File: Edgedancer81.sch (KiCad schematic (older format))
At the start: 17 parts, among them SW1 SW_Push, SW2 Rotary_Encoder_Switch, U1 ATmega32U4-AU, Y1 16MHz

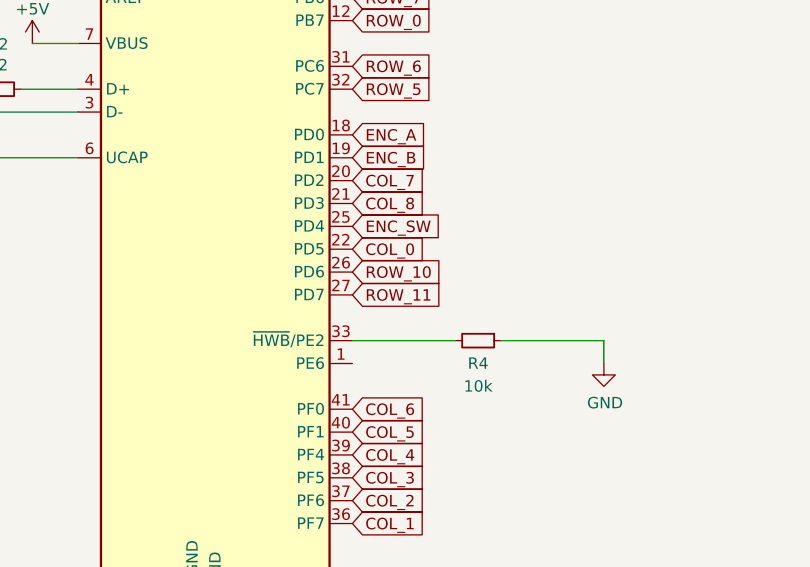
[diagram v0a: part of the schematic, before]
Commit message: silkscreen and bugfixes
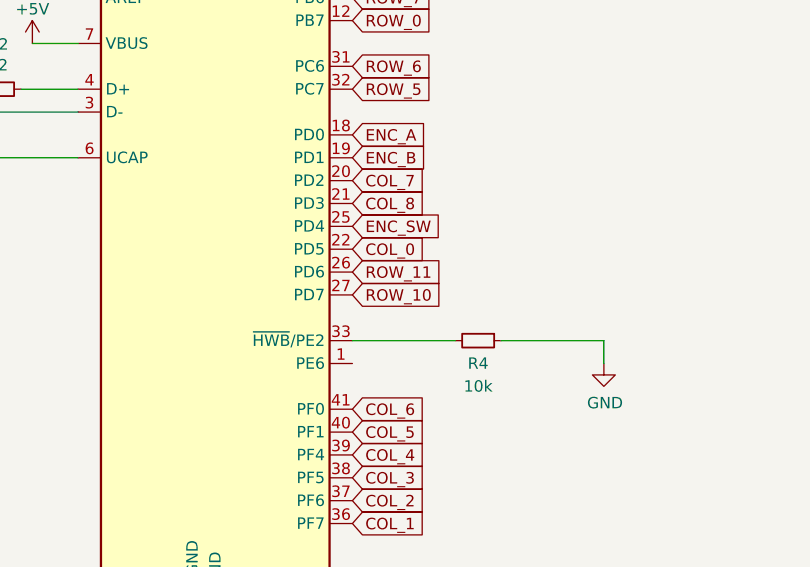
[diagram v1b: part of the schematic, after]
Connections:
- net ROW_10: now also U1.27 (PD7); no longer U1.26 (PD6)
- net ROW_11: now also U1.26 (PD6); no longer U1.27 (PD7)
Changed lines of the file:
@@
 Text GLabel 4050 4000 2    50   Input ~ 0
 ROW_8
+Text GLabel 4050 5400 2    50   Input ~ 0
+ROW_10
 Text GLabel 4050 5300 2    50   Input ~ 0
-ROW_10
-Text GLabel 4050 5400 2    50   Input ~ 0
 ROW_11
 Text GLabel 4050 5100 2    50   Input ~ 0
